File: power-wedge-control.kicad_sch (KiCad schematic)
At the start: 67 parts, among them J1 Conn_01x02, J2 Conn_01x03, J3 Conn_01x02, J4 Conn_01x03, J5 Conn_01x03, J6 Conn_01x06_Female, J7 Conn_01x04_Female, J8 Conn_01x04, J9 MicroSD_Hirose_DM3D-SF, Q1 MMBT3904L, Q2 DMP3099L, Q3 MMBT3904L, Q4 DMP3099L, Q5 MMBT3904L, Q6 MMBT3904L, Q7 MMBT3904L, Q8 MMBT3904L, U1 LM1117-5.0, U3 TLV70233DBV, U4 4050, U5 NC7WZ17P6X, U6 NC7WZ17P6X

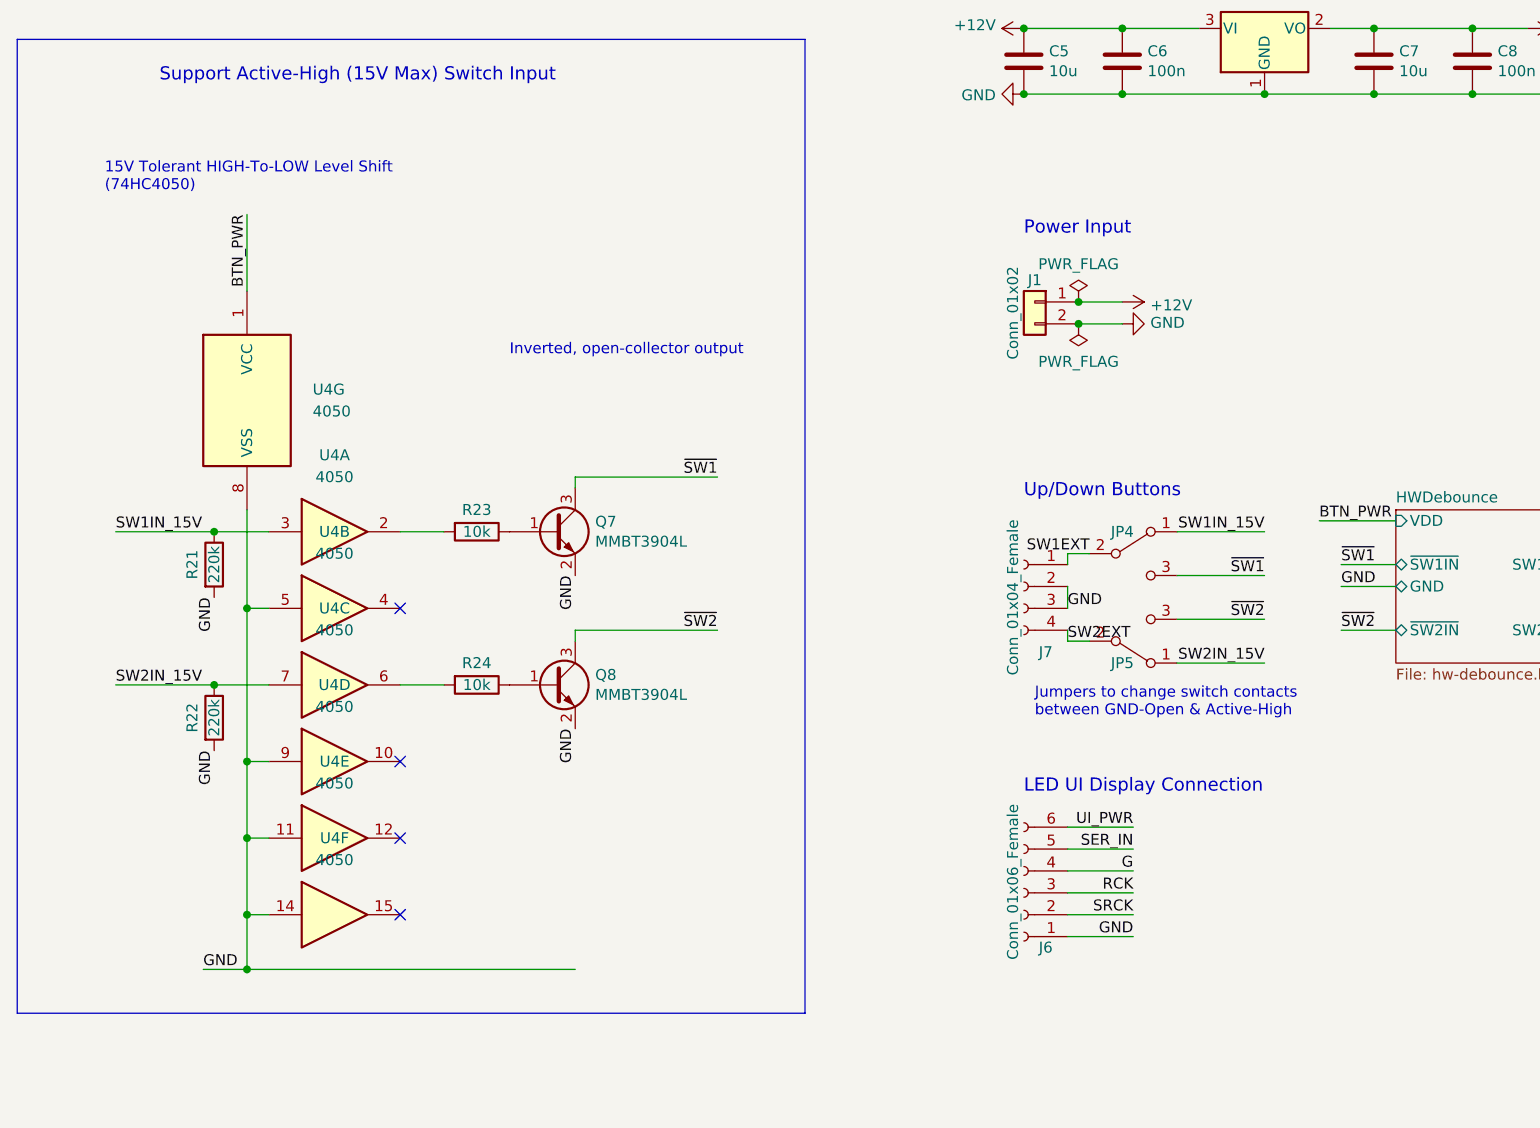
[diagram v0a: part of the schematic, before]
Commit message: Switch to optocouplers, remove GND-Open option for up/down switch input.
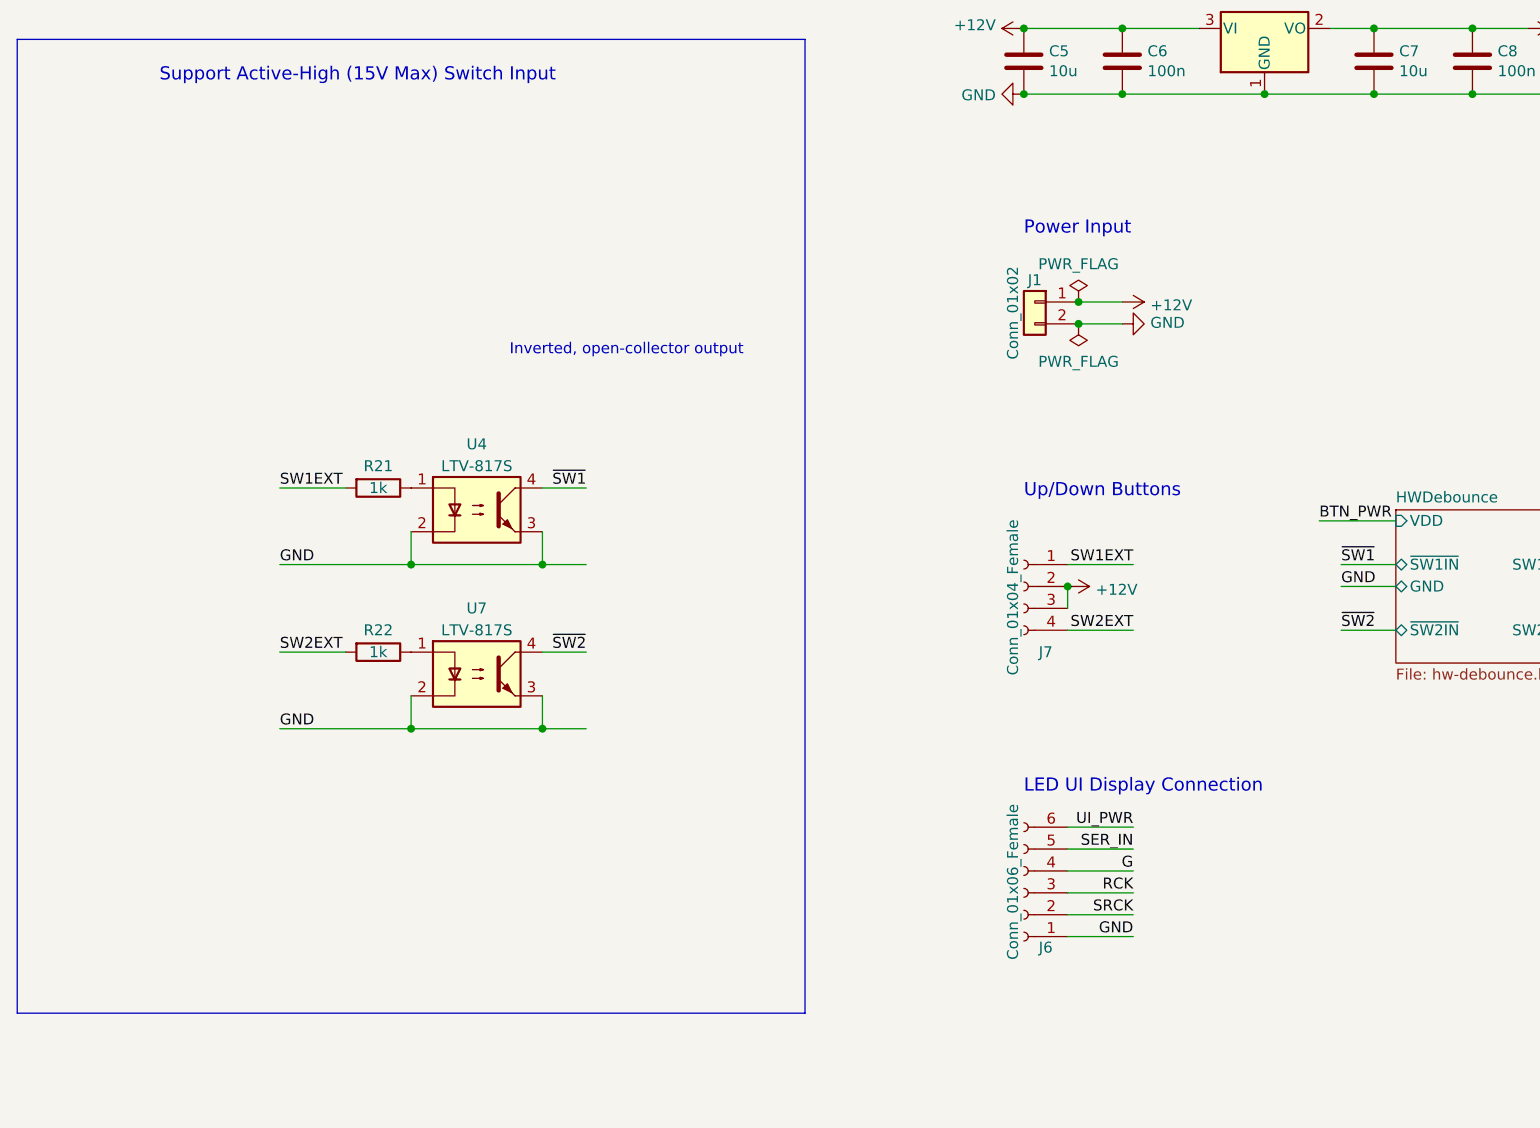
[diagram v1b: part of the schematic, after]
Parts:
- removed JP4, JP5: SW_SPDT, Jumper:SolderJumper-3_P2.0mm_Open_TrianglePad1.0x1.5mm, symbol Switch:SW_SPDT
- removed Q7, Q8: MMBT3904L, Package_TO_SOT_SMD:SOT-23, symbol Device:Q_NPN_BEC
- removed R23, R24: 10k, Resistor_SMD:R_0603_1608Metric, symbol Device:R
- removed U4: 4050, Package_SO:SOIC-16W_5.3x10.2mm_P1.27mm, symbol 4xxx:4050
- added U4, U7: LTV-817S, Package_DIP:SMDIP-4_W9.53mm, symbol Isolator:LTV-817S
- R21, R22: value 220k -> 1k
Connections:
- net +12V: now also J7.2 (Pin_2), J7.3 (Pin_3)
- net GND: now also U4.2, U4.3, U7.2, U7.3; no longer J7.2 (Pin_2), J7.3 (Pin_3), R21.2, R22.2
- net SW1EXT: now also R21.2
- net SW2EXT: now also R22.2
- net ~{SW1}: now also U4.4
- net ~{SW2}: now also U7.4
- net SW1IN_15V: no longer names the net of R21.1
- net SW1IN_15V: now also U4.1
- net SW2IN_15V: no longer names the net of R22.1
- net SW2IN_15V: now also U7.1
- no-connect marks 47 -> 43
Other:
- note removed: "15V Tolerant HIGH-To-LOW Level Shift (74HC4050)"
- note removed: "Jumpers to change switch contacts between GND-Open & Active-High"

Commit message: Exclude Adafruit Huzzah32 ESP32 from board/bom.
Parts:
- A2: now left out of the parts list
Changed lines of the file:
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@@
   )
   (symbol (lib_id "MCU_Module:Adafruit_Feather_HUZZAH32_ESP32") (at 177.8 50.8 0) (unit 1)
-    (in_bom yes) (on_board yes) (fields_autoplaced)
+    (in_bom no) (on_board no) (fields_autoplaced)
     (property "Reference" "A2" (id 0) (at 179.8194 83.82 0)
       (effects (font (size 1.27 1.27)) (justify left))
